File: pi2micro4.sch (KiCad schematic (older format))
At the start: 17 parts, among them M1 microduino_base, M2 microduino_base, M3 microduino_base, M4 microduino_base, P1 CONN_13X2, U1 NCP1117ST33T3G, U2 txs0104e

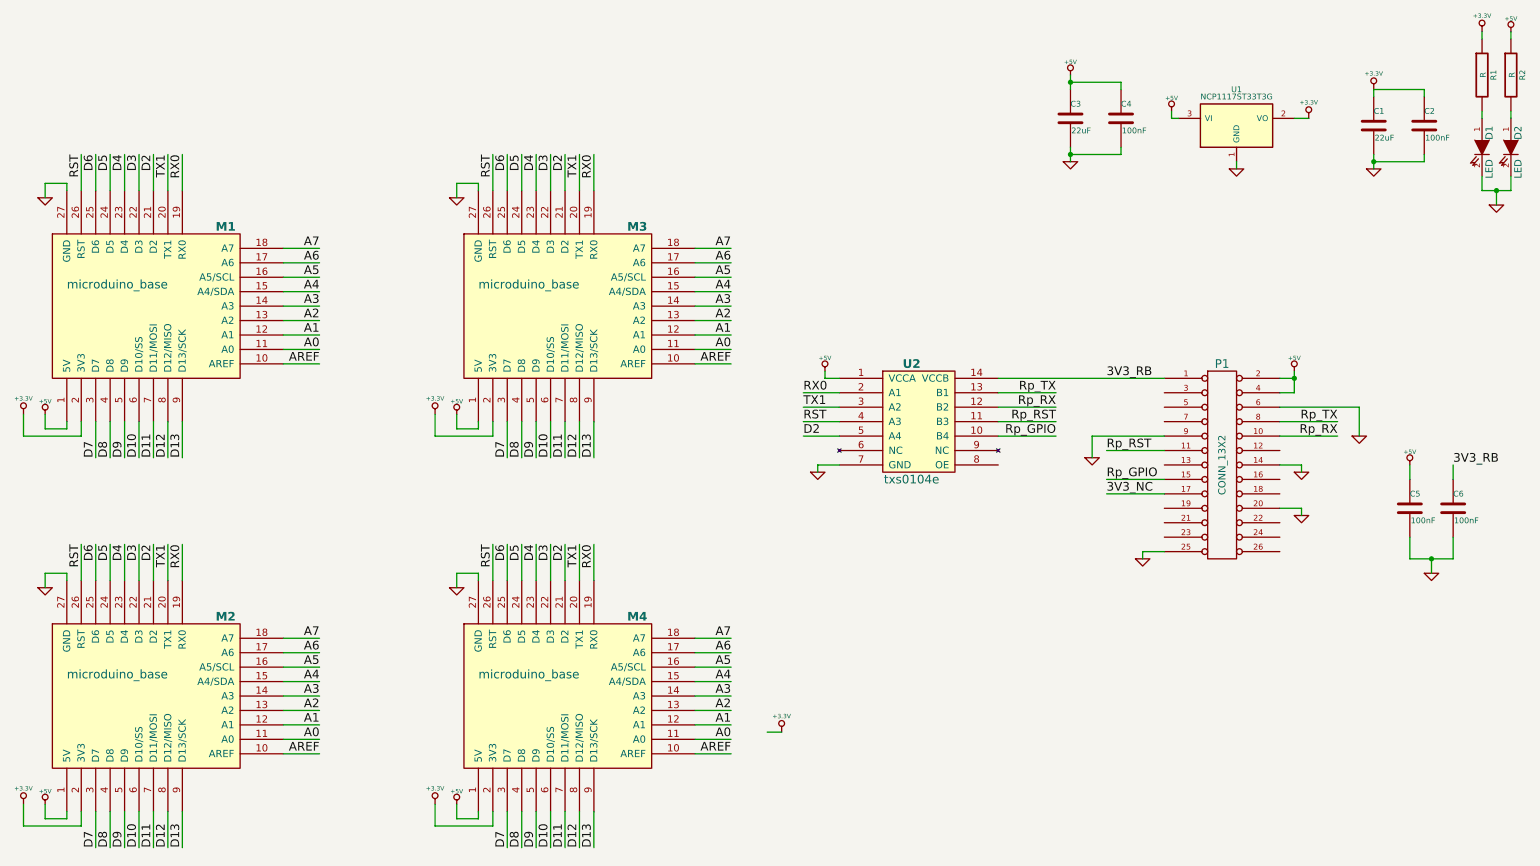
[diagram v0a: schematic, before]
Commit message: nuevo buffer
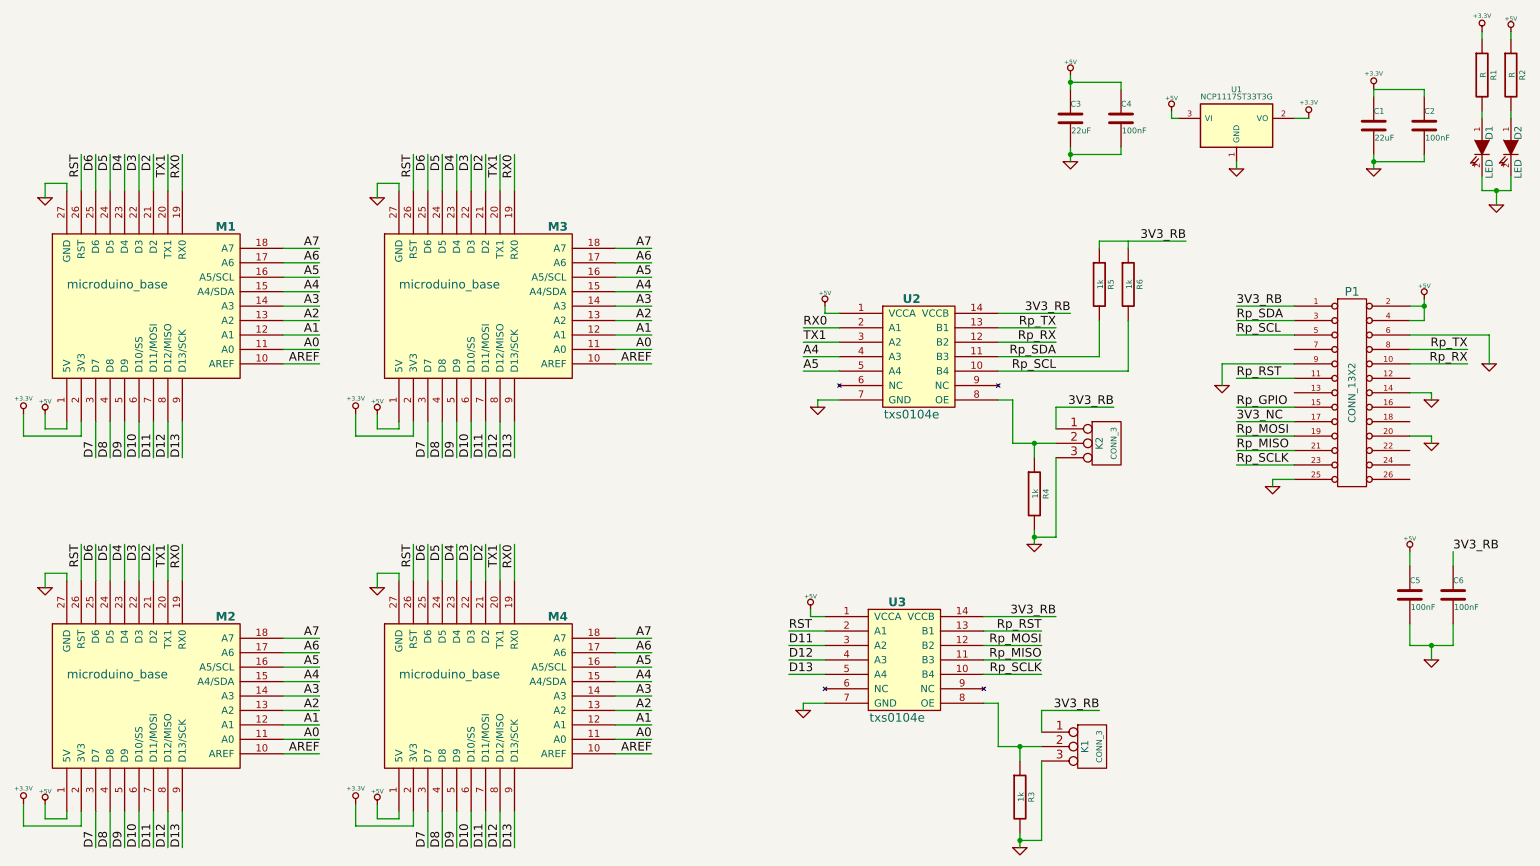
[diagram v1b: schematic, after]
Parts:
- added K1, K2: CONN_3, SIL-3, symbol CONN_3
- added R3, R4, R5, R6: 1k, SMD-0603, symbol R
- added U3: txs0104e, TSSOP-14, symbol txs0104e
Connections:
- net +5V: now also U3.1 (VCCA)
- net 3V3_RB: now also K1.1 (P1), K2.1 (P1), R5.1, U3.14 (VCCB)
- net A4: now also U2.4 (A3)
- net A5: now also U2.5 (A4)
- net D11: now also U3.3 (A2)
- net D12: now also U3.4 (A3)
- net D13: now also U3.5 (A4)
- net D2: no longer U2.5 (A4)
- net GND: now also K1.3 (P3), K2.3 (P3), R3.2, R4.2, U3.7 (GND)
- net RST: now also U3.2 (A1); no longer U2.4 (A3)
- net Rp_GPIO: no longer U2.10 (B4)
- net Rp_RST: now also U3.13 (B1); no longer U2.11 (B3)
- net Rp_MOSI: now reaches P1.19 (P19)
- net Rp_MOSI: now also U3.12 (B2)
- net Rp_MISO: now reaches P1.21 (P21)
- net Rp_MISO: now also U3.11 (B3)
- net Rp_SCLK: now reaches P1.23 (P23)
- net Rp_SCLK: now also U3.10 (B4)
- net Rp_SDA: now reaches P1.3 (P3)
- net Rp_SDA: now also U2.11 (B3), R5.2
- net Rp_SCL: now reaches P1.5 (P5)
- net Rp_SCL: now also U2.10 (B4), R6.2
- net at U2.8 (OE): now also K2.2 (PM), R4.1
- new net: K1.2 (PM), R3.1, U3.8 (OE)
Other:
- moved on the sheet: C5, C6, M3, M4, P1, U2
